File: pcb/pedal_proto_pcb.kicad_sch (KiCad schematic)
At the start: 18 parts, among them J1 100k_pot_1, J10 100k_pot_2, J11 250k_pot_1, J12 250k_pot_2, J13 stomp_b, J14 stomp_a, J15 stomp_c, J16 switch, J17 LED, J18 LED, J2 100k_pot_2, J3 250k_pot_1, J4 250k_pot_2, J5 stomp, J6 switch, J7 power, J8 LED, J9 100k_pot_1

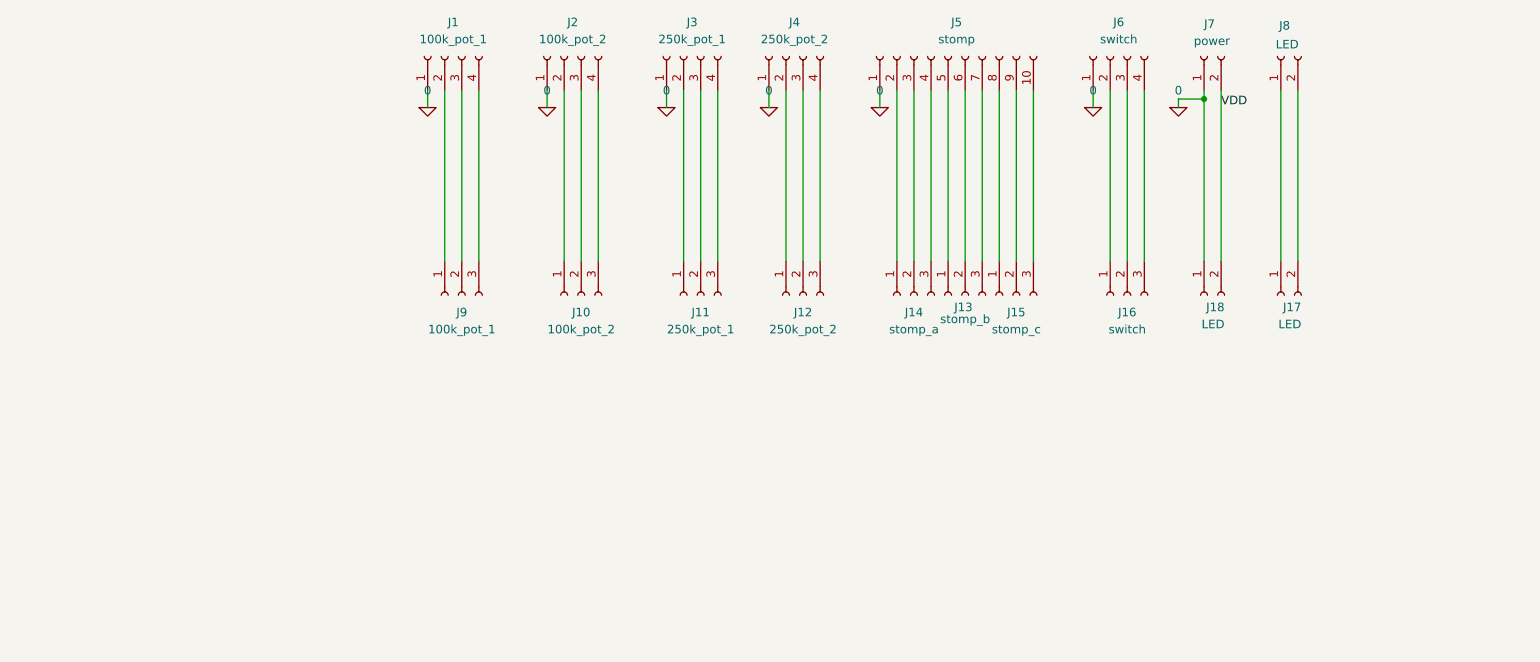
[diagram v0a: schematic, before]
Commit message: feat: pcb done
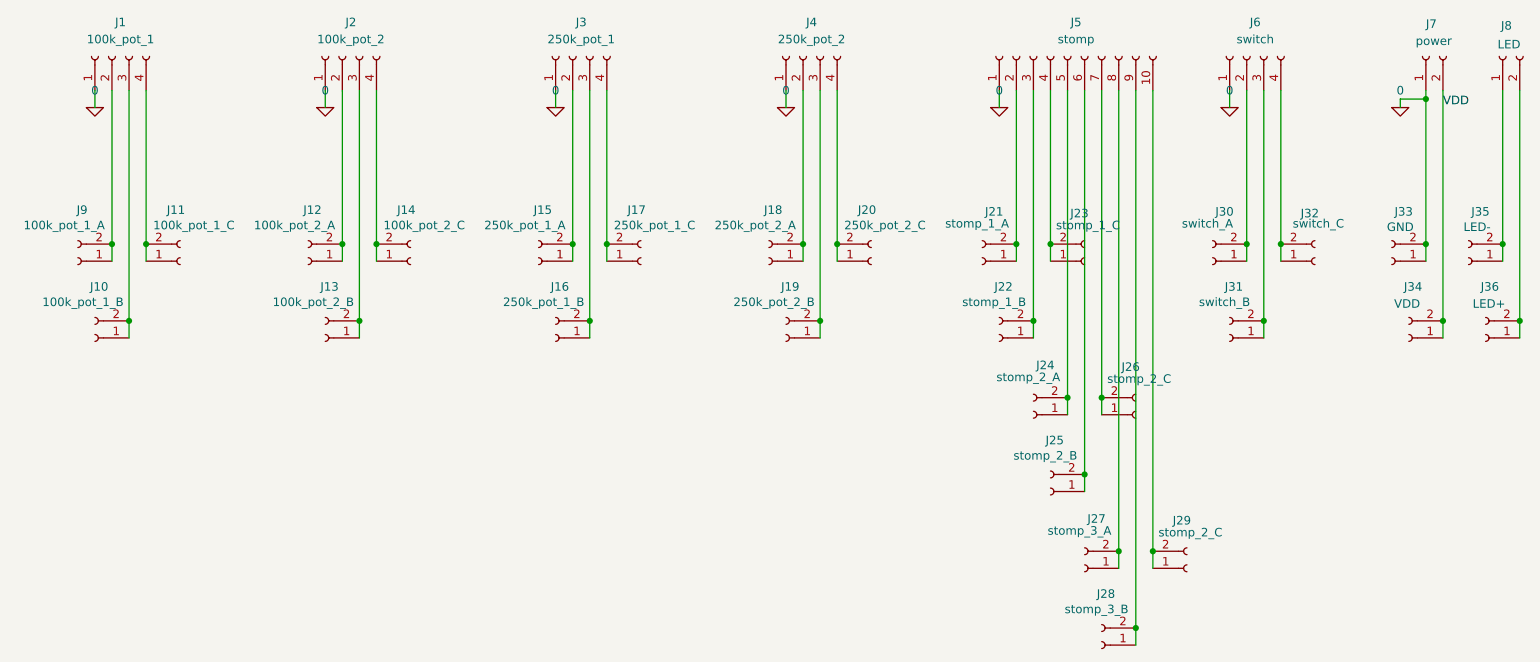
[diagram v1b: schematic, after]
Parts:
- removed J10: 100k_pot_2, symbol Connector:Conn_01x03_Socket
- removed J11: 250k_pot_1, symbol Connector:Conn_01x03_Socket
- removed J12: 250k_pot_2, symbol Connector:Conn_01x03_Socket
- removed J13: stomp_b, symbol Connector:Conn_01x03_Socket
- removed J14: stomp_a, symbol Connector:Conn_01x03_Socket
- removed J15: stomp_c, symbol Connector:Conn_01x03_Socket
- removed J16: switch, symbol Connector:Conn_01x03_Socket
- removed J9: 100k_pot_1, symbol Connector:Conn_01x03_Socket
- added J10: 100k_pot_1_B, Connector_PinHeader_2.54mm:PinHeader_1x02_P2.54mm_Vertical, symbol Connector:Conn_01x02_Socket
- added J11: 100k_pot_1_C, Connector_PinHeader_2.54mm:PinHeader_1x02_P2.54mm_Vertical, symbol Connector:Conn_01x02_Socket
- added J12: 100k_pot_2_A, Connector_PinHeader_2.54mm:PinHeader_1x02_P2.54mm_Vertical, symbol Connector:Conn_01x02_Socket
- added J13: 100k_pot_2_B, Connector_PinHeader_2.54mm:PinHeader_1x02_P2.54mm_Vertical, symbol Connector:Conn_01x02_Socket
- added J14: 100k_pot_2_C, Connector_PinHeader_2.54mm:PinHeader_1x02_P2.54mm_Vertical, symbol Connector:Conn_01x02_Socket
- added J15: 250k_pot_1_A, Connector_PinHeader_2.54mm:PinHeader_1x02_P2.54mm_Vertical, symbol Connector:Conn_01x02_Socket
- added J16: 250k_pot_1_B, Connector_PinHeader_2.54mm:PinHeader_1x02_P2.54mm_Vertical, symbol Connector:Conn_01x02_Socket
- added J19: 250k_pot_2_B, Connector_PinHeader_2.54mm:PinHeader_1x02_P2.54mm_Vertical, symbol Connector:Conn_01x02_Socket
- added J20: 250k_pot_2_C, Connector_PinHeader_2.54mm:PinHeader_1x02_P2.54mm_Vertical, symbol Connector:Conn_01x02_Socket
- added J21: stomp_1_A, Connector_PinHeader_2.54mm:PinHeader_1x02_P2.54mm_Vertical, symbol Connector:Conn_01x02_Socket
- added J22: stomp_1_B, Connector_PinHeader_2.54mm:PinHeader_1x02_P2.54mm_Vertical, symbol Connector:Conn_01x02_Socket
- added J23: stomp_1_C, Connector_PinHeader_2.54mm:PinHeader_1x02_P2.54mm_Vertical, symbol Connector:Conn_01x02_Socket
- added J24: stomp_2_A, Connector_PinHeader_2.54mm:PinHeader_1x02_P2.54mm_Vertical, symbol Connector:Conn_01x02_Socket
- added J25: stomp_2_B, Connector_PinHeader_2.54mm:PinHeader_1x02_P2.54mm_Vertical, symbol Connector:Conn_01x02_Socket
- added J26, J29: stomp_2_C, Connector_PinHeader_2.54mm:PinHeader_1x02_P2.54mm_Vertical, symbol Connector:Conn_01x02_Socket
- added J27: stomp_3_A, Connector_PinHeader_2.54mm:PinHeader_1x02_P2.54mm_Vertical, symbol Connector:Conn_01x02_Socket
- added J28: stomp_3_B, Connector_PinHeader_2.54mm:PinHeader_1x02_P2.54mm_Vertical, symbol Connector:Conn_01x02_Socket
- added J30: switch_A, Connector_PinHeader_2.54mm:PinHeader_1x02_P2.54mm_Vertical, symbol Connector:Conn_01x02_Socket
- added J31: switch_B, Connector_PinHeader_2.54mm:PinHeader_1x02_P2.54mm_Vertical, symbol Connector:Conn_01x02_Socket
- added J32: switch_C, Connector_PinHeader_2.54mm:PinHeader_1x02_P2.54mm_Vertical, symbol Connector:Conn_01x02_Socket
- added J33: GND, Connector_PinHeader_2.54mm:PinHeader_1x02_P2.54mm_Vertical, symbol Connector:Conn_01x02_Socket
- added J34: VDD, Connector_PinHeader_2.54mm:PinHeader_1x02_P2.54mm_Vertical, symbol Connector:Conn_01x02_Socket
- added J35: LED-, Connector_PinHeader_2.54mm:PinHeader_1x02_P2.54mm_Vertical, symbol Connector:Conn_01x02_Socket
- added J36: LED+, Connector_PinHeader_2.54mm:PinHeader_1x02_P2.54mm_Vertical, symbol Connector:Conn_01x02_Socket
- added J9: 100k_pot_1_A, Connector_PinHeader_2.54mm:PinHeader_1x02_P2.54mm_Vertical, symbol Connector:Conn_01x02_Socket
- J1, J2, J3, J4, J6: footprint (none) -> Connector_PinHeader_2.54mm:PinHeader_1x04_P2.54mm_Vertical
- J17: value LED -> 250k_pot_1_C; footprint (none) -> Connector_PinHeader_2.54mm:PinHeader_1x02_P2.54mm_Vertical
- J18: value LED -> 250k_pot_2_A; footprint (none) -> Connector_PinHeader_2.54mm:PinHeader_1x02_P2.54mm_Vertical
- J5: footprint (none) -> Connector_PinHeader_2.54mm:PinHeader_1x10_P2.54mm_Vertical
- J7, J8: footprint (none) -> Connector_PinHeader_2.54mm:PinHeader_1x02_P2.54mm_Vertical
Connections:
- net 0: now also J33.1 (Pin_1), J33.2 (Pin_2); no longer J18.1 (Pin_1)
- net VDD: now also J34.1 (Pin_1), J34.2 (Pin_2); no longer J18.2 (Pin_2)
- net at J6.2 (Pin_2): now also J30.1 (Pin_1), J30.2 (Pin_2)
- net at J6.3 (Pin_3): now also J31.1 (Pin_1), J31.2 (Pin_2)
- net at J6.4 (Pin_4): now also J32.1 (Pin_1), J32.2 (Pin_2)
- net at J5.5 (Pin_5): now also J24.1 (Pin_1), J24.2 (Pin_2)
- net at J5.6 (Pin_6): now also J25.1 (Pin_1), J25.2 (Pin_2)
- net at J5.7 (Pin_7): now also J26.1 (Pin_1), J26.2 (Pin_2)
- net at J2.2 (Pin_2): now also J12.1 (Pin_1), J12.2 (Pin_2)
- net at J2.3 (Pin_3): now also J13.1 (Pin_1), J13.2 (Pin_2)
- net at J2.4 (Pin_4): now also J14.1 (Pin_1), J14.2 (Pin_2)
- net at J5.10 (Pin_10): now also J29.1 (Pin_1), J29.2 (Pin_2)
- net at J5.2 (Pin_2): now also J21.1 (Pin_1), J21.2 (Pin_2)
- net at J5.3 (Pin_3): now also J22.1 (Pin_1), J22.2 (Pin_2)
- net at J5.4 (Pin_4): now also J23.1 (Pin_1), J23.2 (Pin_2)
- net at J5.8 (Pin_8): now also J27.1 (Pin_1), J27.2 (Pin_2)
- net at J5.9 (Pin_9): now also J28.1 (Pin_1), J28.2 (Pin_2)
- net at J1.2 (Pin_2): now also J9.1 (Pin_1), J9.2 (Pin_2)
- net at J1.3 (Pin_3): now also J10.1 (Pin_1), J10.2 (Pin_2)
- net at J1.4 (Pin_4): now also J11.1 (Pin_1), J11.2 (Pin_2)
- net at J4.2 (Pin_2): now also J18.1 (Pin_1), J18.2 (Pin_2)
- net at J4.3 (Pin_3): now also J19.1 (Pin_1), J19.2 (Pin_2)
- net at J4.4 (Pin_4): now also J20.1 (Pin_1), J20.2 (Pin_2)
- net at J3.2 (Pin_2): now also J15.1 (Pin_1), J15.2 (Pin_2)
- net at J3.3 (Pin_3): now also J16.1 (Pin_1), J16.2 (Pin_2)
- net at J3.4 (Pin_4): now also J17.1 (Pin_1), J17.2 (Pin_2)
- net at J8.1 (Pin_1): now also J35.1 (Pin_1), J35.2 (Pin_2); no longer J17.1 (Pin_1)
- net at J8.2 (Pin_2): now also J36.1 (Pin_1), J36.2 (Pin_2); no longer J17.2 (Pin_2)
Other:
- moved on the sheet: J1, J2, J3, J4, J5, J6, J7, J8
